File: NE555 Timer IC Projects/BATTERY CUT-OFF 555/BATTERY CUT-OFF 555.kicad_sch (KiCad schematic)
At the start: 19 parts, among them J1 BATTERY, J2 CHARGE INPUT, K1 SANYOU_SRD_Form_A, Q1 AO3400A, U1 LM555xM, U2 LM393

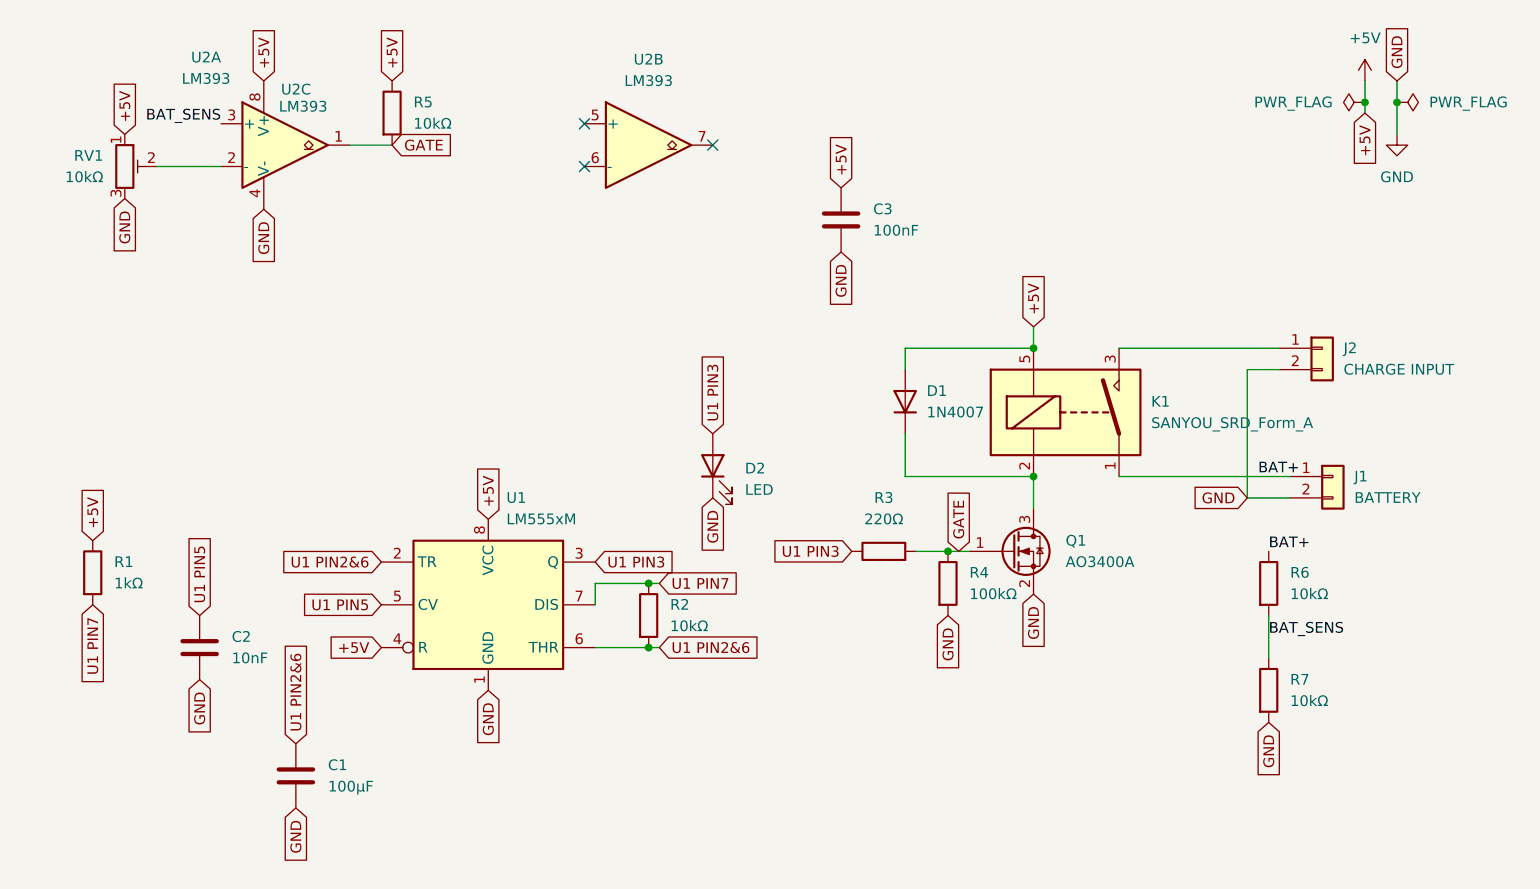
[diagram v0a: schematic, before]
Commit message: Initial Commit
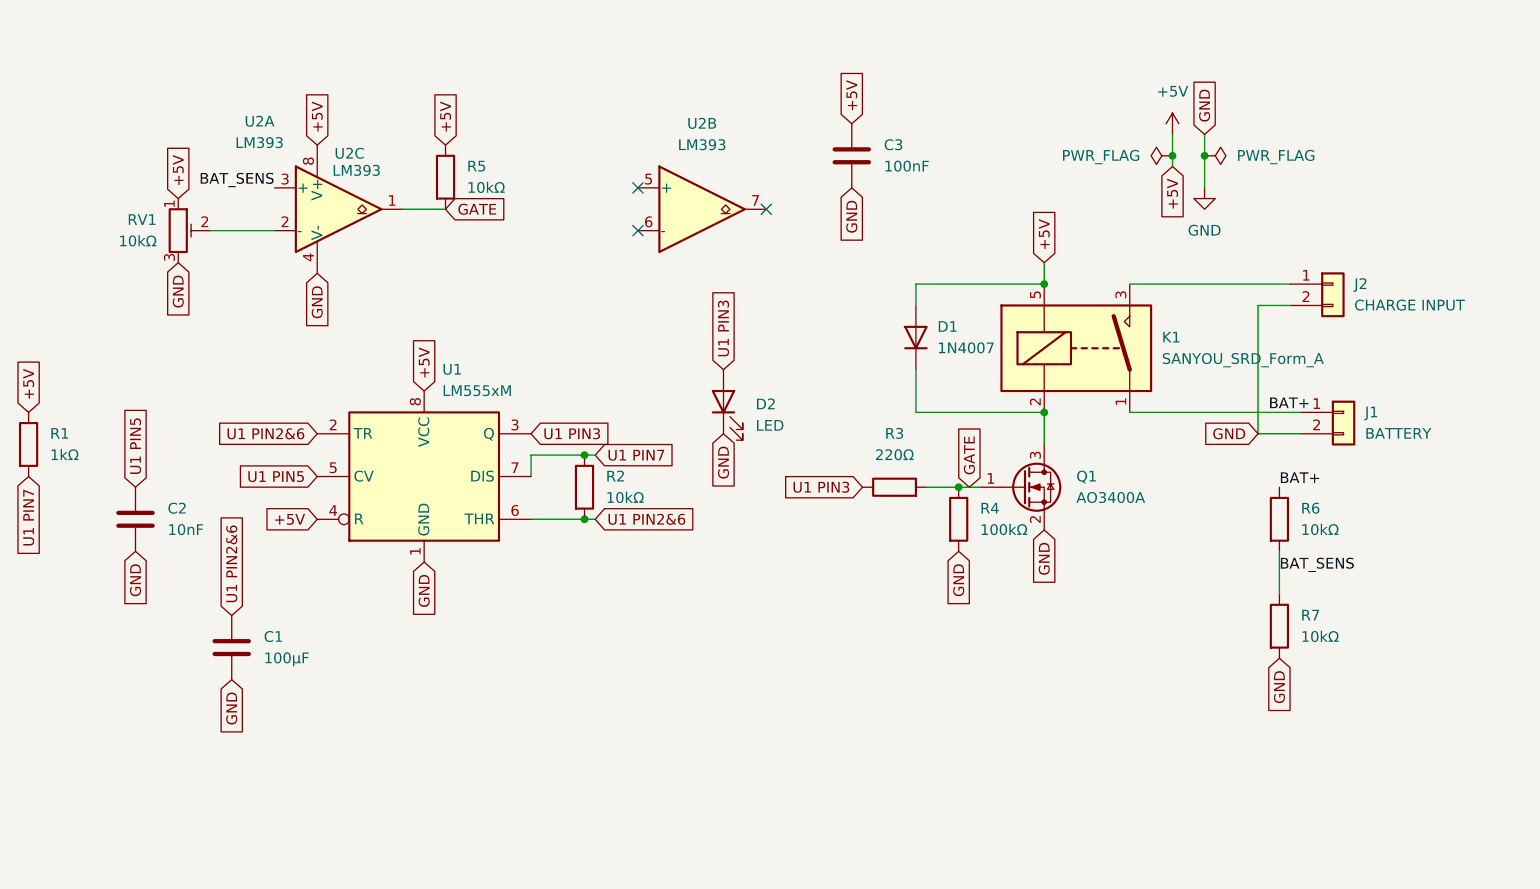
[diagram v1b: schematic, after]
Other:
- moved on the sheet: C1, C2, C3, D1, D2, J1, J2, K1, Q1, R1, R2, R3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
